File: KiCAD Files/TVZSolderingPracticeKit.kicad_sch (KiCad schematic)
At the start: 22 parts, among them SW1 SW_Push, SW10 SW_SPDT, SW2 SW_Push, SW3 SW_Push, SW4 SW_Push, SW5 SW_Push, SW6 SW_Push, SW7 SW_Push, SW8 SW_Push, U1 NE555P

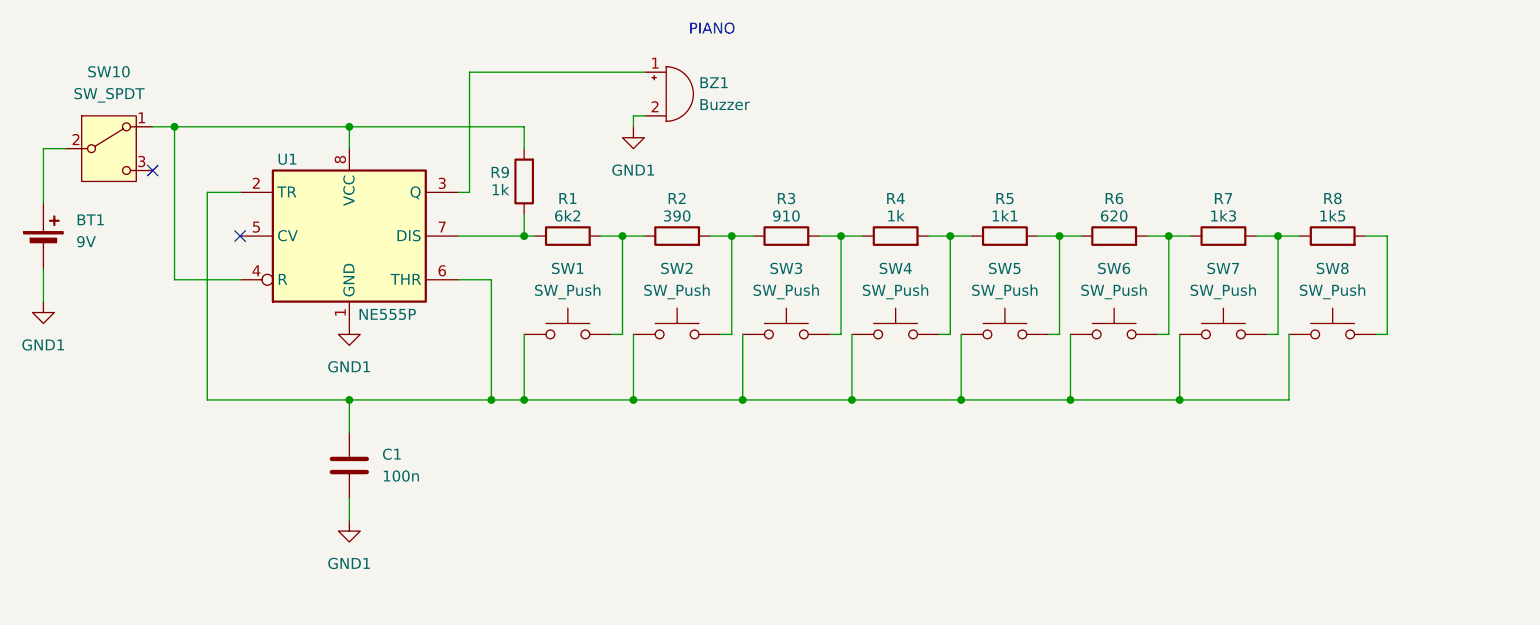
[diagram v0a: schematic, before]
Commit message: update
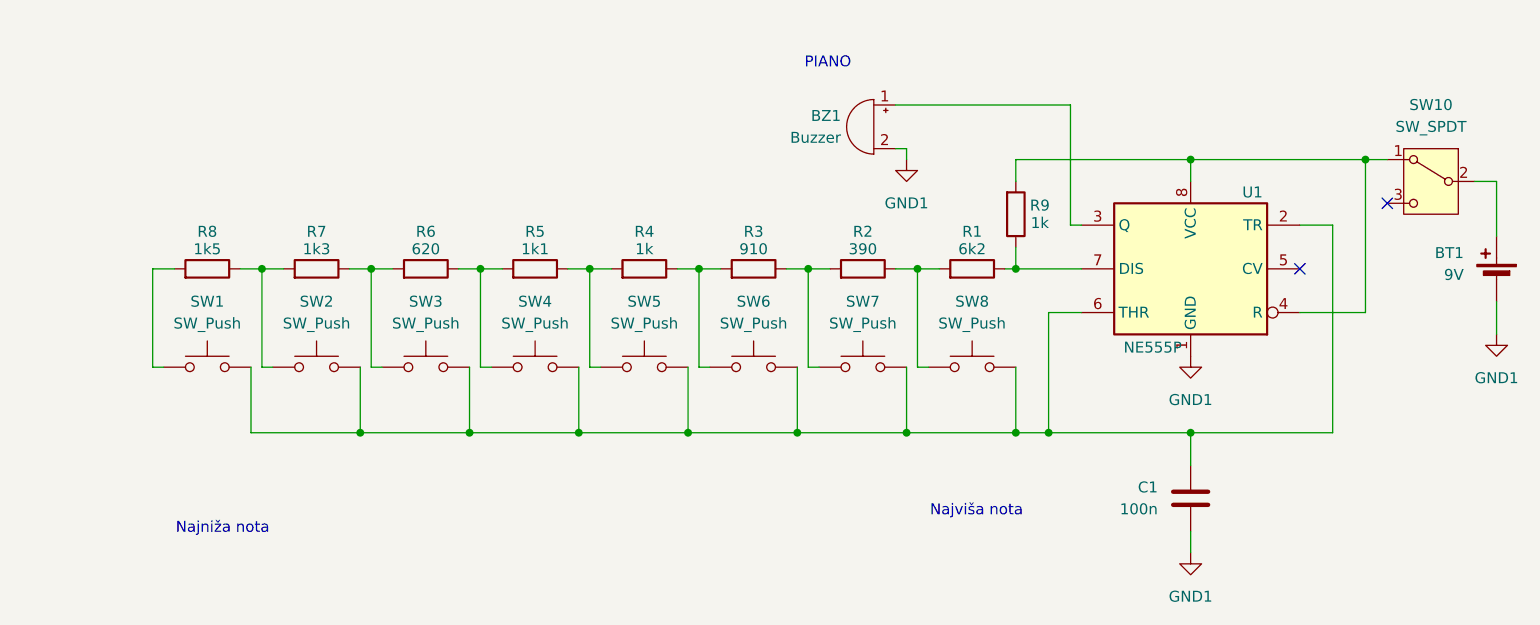
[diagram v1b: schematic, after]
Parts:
- R1, R2, R3, R4, R5, R6, R7, R8, R9: footprint Resistor_THT:R_Axial_DIN0207_L6.3mm_D2.5mm_P7.62mm_Horizontal -> Resistor_THT:R_Axial_DIN0207_L6.3mm_D2.5mm_P10.16mm_Horizontal
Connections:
- net at R7.2, R8.1: now also SW2.1; no longer SW7.2
- net at R8.2: now also SW1.1; no longer SW8.2
- net at R3.2, R4.1: now also SW6.1; no longer SW3.2
- net at R1.2, R2.1: now also SW8.1; no longer SW1.2
- net at R2.2, R3.1: now also SW7.1; no longer SW2.2
- net at R5.2, R6.1: now also SW4.1; no longer SW5.2
- net at R6.2, R7.1: now also SW3.1; no longer SW6.2
- net at R4.2, R5.1: now also SW5.1; no longer SW4.2
- new net: C1.1, SW1.2, SW2.2, SW3.2, SW4.2, SW5.2, SW6.2, SW7.2, SW8.2, U1.2 (TR), U1.6 (THR)
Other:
- note added: "Najniža nota"
- note added: "Najviša nota"
- moved on the sheet: BT1, BZ1, C1, R1, R2, R3, R4, R5, R6, R7, R8, R9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
